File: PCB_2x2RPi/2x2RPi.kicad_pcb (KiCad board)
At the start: 2 copper layers, 44.5 x 53.3 mm, 31 parts, among them J1 USB, P1 VIN, P2 CONN_13X2, P3 INPUT, P4 REL2, P5 5V, P6 REL1, SW1 PWR SW, U1 LowCurVReg, U2 LowCurVReg, U3 TLP2531, U4 INVERTER-1CH, U5 INVERTER-1CH

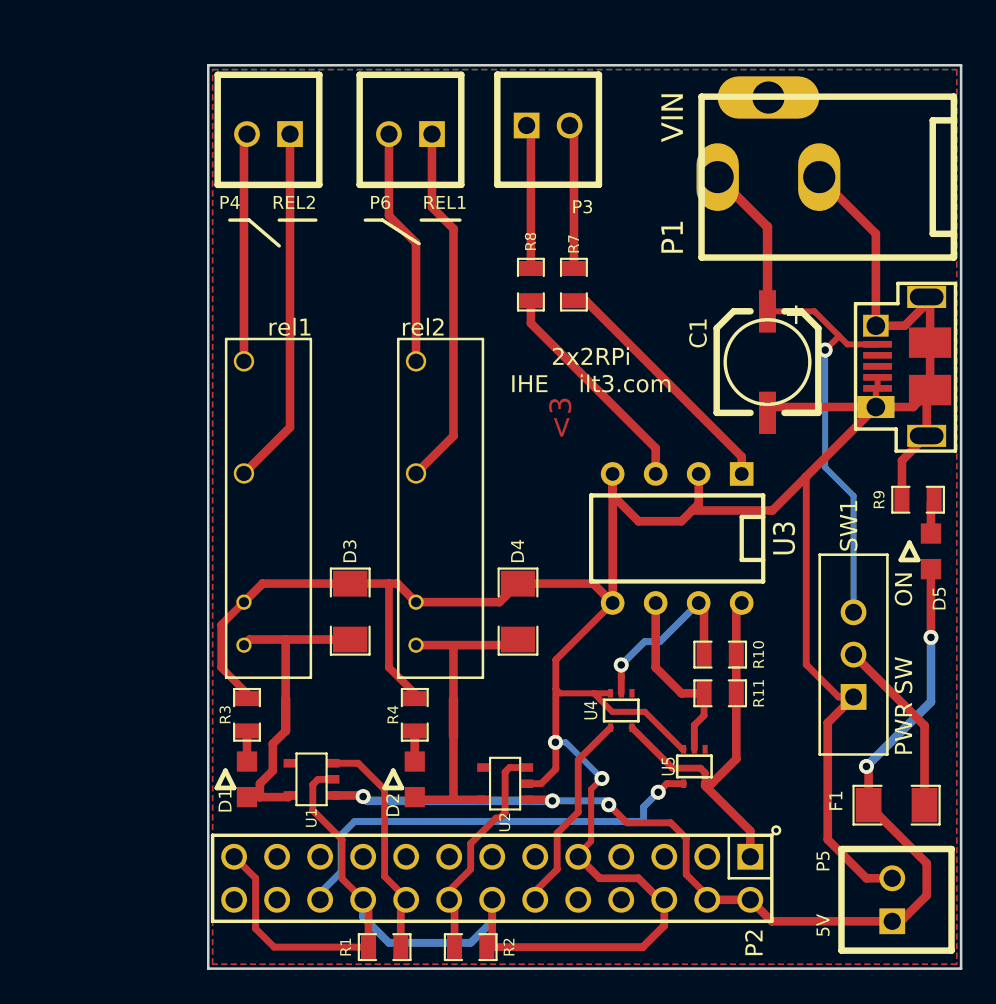
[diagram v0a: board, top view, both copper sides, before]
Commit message: 2nd revision 2x2RPi board and gerber files, awaiting approval
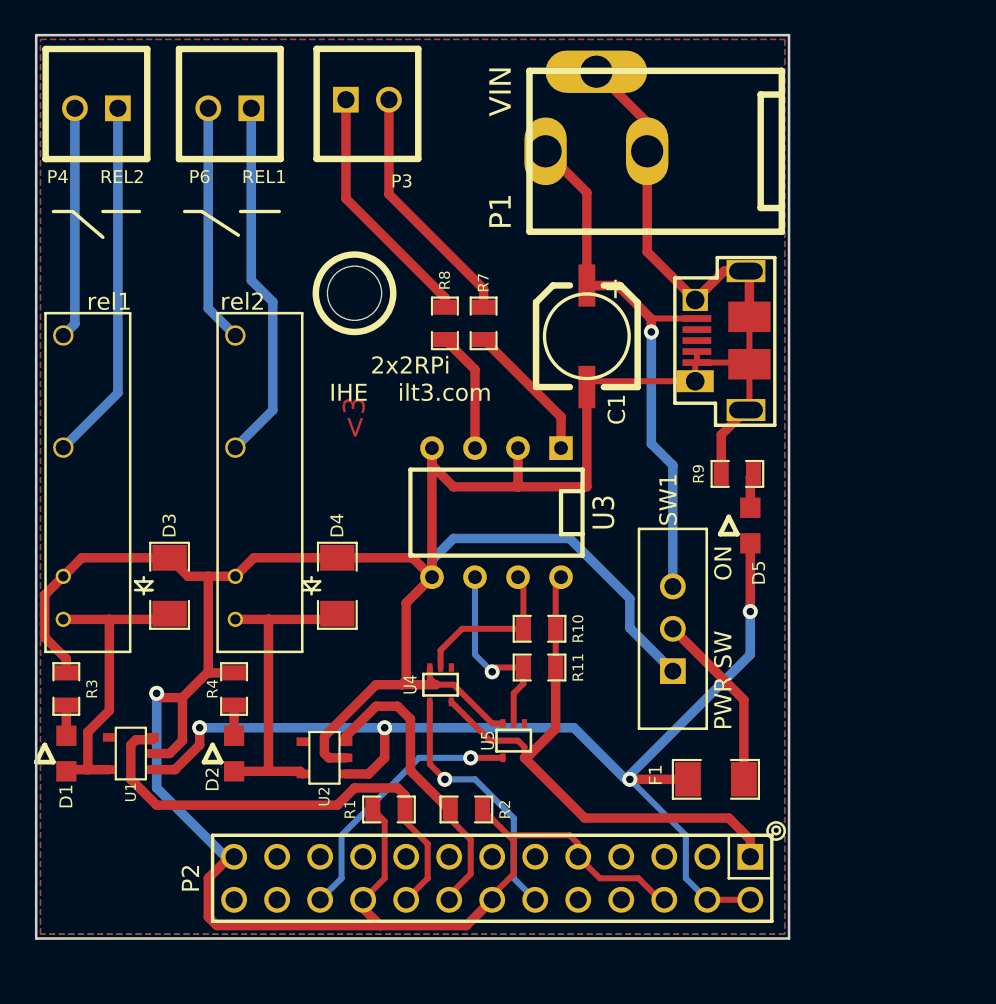
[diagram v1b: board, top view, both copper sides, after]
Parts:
- removed P5: 5V, PIN_ARRAY_2X1_Screw Terminal
- added 1PIN: P***, 1pin_NPTH_Mechanical_M3_Screw, F.Cu at (110.2, 64.3)
- moved D2 10.8 mm to (103.1, 91.4)
- moved D3 10.8 mm to (99.3, 81.5)
- moved D4 10.8 mm to (109.2, 81.5)
- moved F1 10.8 mm to (131.6, 93.0)
- moved J1 10.8 mm to (133.3, 67.1)
- moved R4 10.8 mm to (103.1, 87.6)
- moved U2 10.8 mm to (108.5, 91.7)
- moved U3 10.8 mm to (118.6, 77.2)
- moved rel1 10.8 mm to (94.5, 75.4)
- moved rel2 10.8 mm to (104.6, 75.4)
- moved C1 10.8 mm to (124.0, 66.8)
- moved D1 10.8 mm to (93.2, 91.4)
- moved P3 10.8 mm to (111.0, 52.8)
- moved R10 10.8 mm to (121.2, 84.1)
- moved R11 10.8 mm to (121.2, 86.4)
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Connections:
- P1 pad 3: (no net) -> GND
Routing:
- net /GPIO_24: track 13.6 -> 28.2 mm
- net /3V3: track 23.3 -> 34.0 mm
- net /GPIO_25: track 26.3 -> 15.8 mm
- net N-0000034: track 14.7 -> 8.31 mm
- net /IN_25: track 8.55 -> 14.7 mm
- net N-0000033: track 13.3 -> 7.15 mm
- net /IN_18: track 8.55 -> 14.6 mm
- net /GPIO_23: track 13.3 -> 17.9 mm
- net GND: track 226.8 -> 222.4 mm, vias 2 -> 1
- net /5V-RPI: track 64.0 -> 67.4 mm, vias 5 -> 4
- net /5Vreg: track 33.8 -> 37.2 mm
- net /GPIO_18: track 12.0 -> 15.3 mm, vias 0 -> 1
- net N-0000032: track 10.9 -> 9.61 mm, vias 1 -> 0
- net /5V-Relay2: track 19.2 -> 18.4 mm
- net N-0000031: track 10.8 -> 11.5 mm, vias 0 -> 1
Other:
- board size 44.5 x 53.3 mm -> 44.4 x 53.3 mm
